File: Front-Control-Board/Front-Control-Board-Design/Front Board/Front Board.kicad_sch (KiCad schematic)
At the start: 27 parts, among them J1 Conn_01x14, J2 Conn_01x14, J3 Conn_01x08, Q1 2N7002, U1 MAX33054EASA+T, U2 TS2940CP33_ROG, U3 ESP32-DevKitC

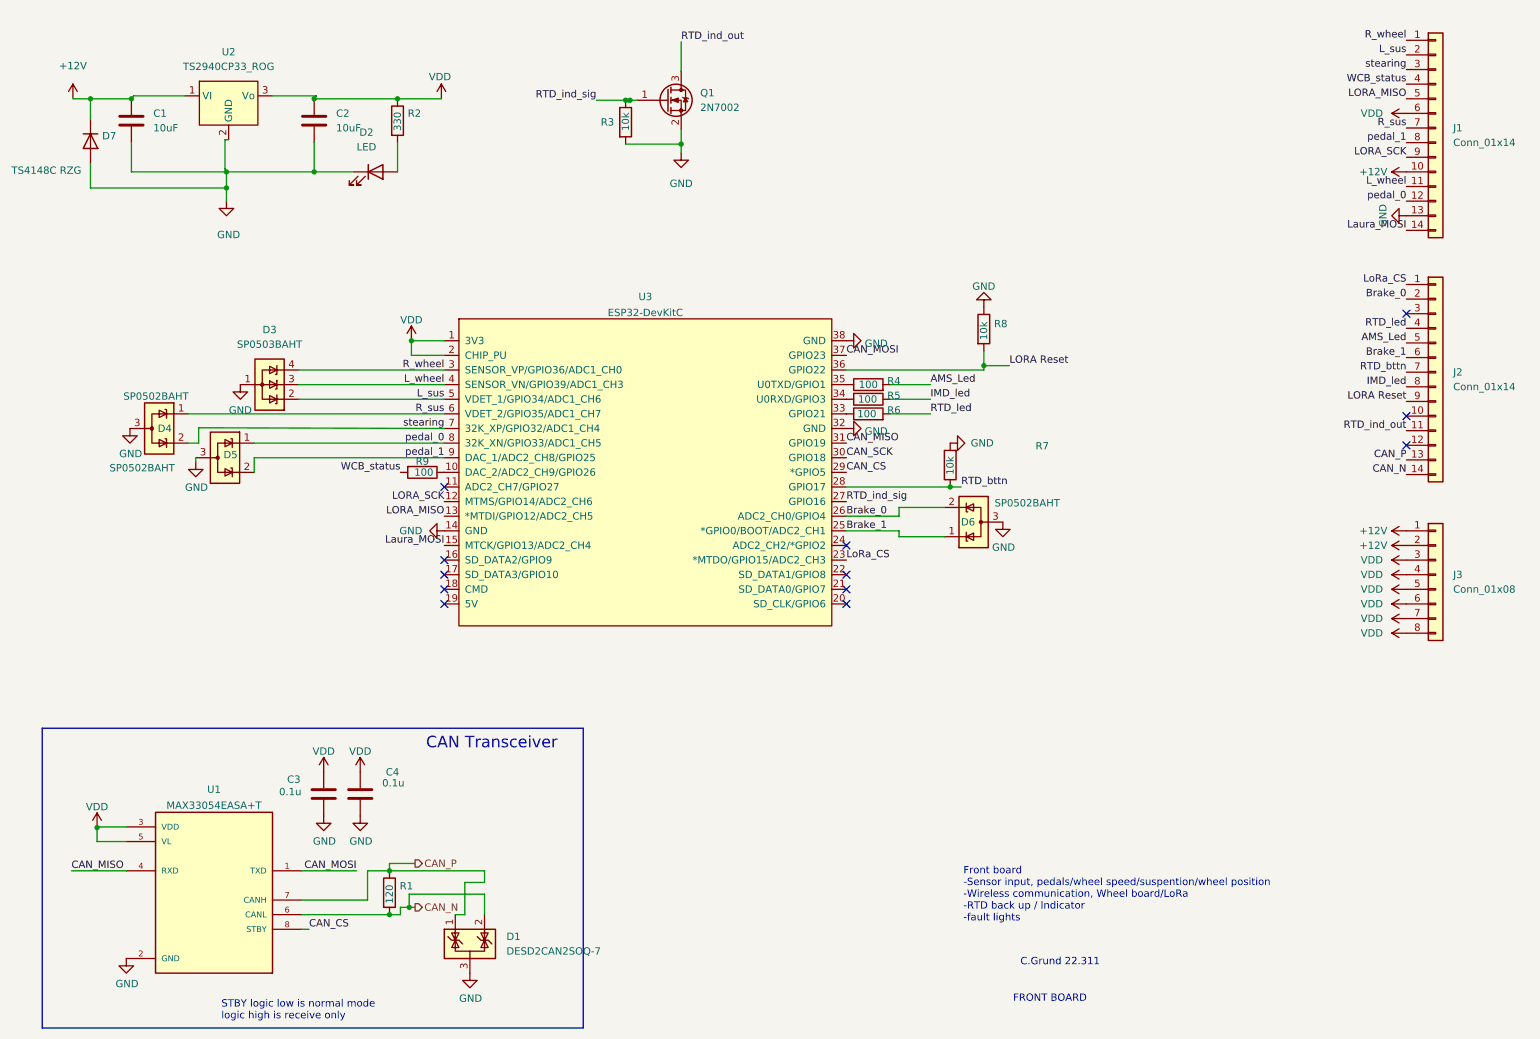
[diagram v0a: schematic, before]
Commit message: end of year DUMP
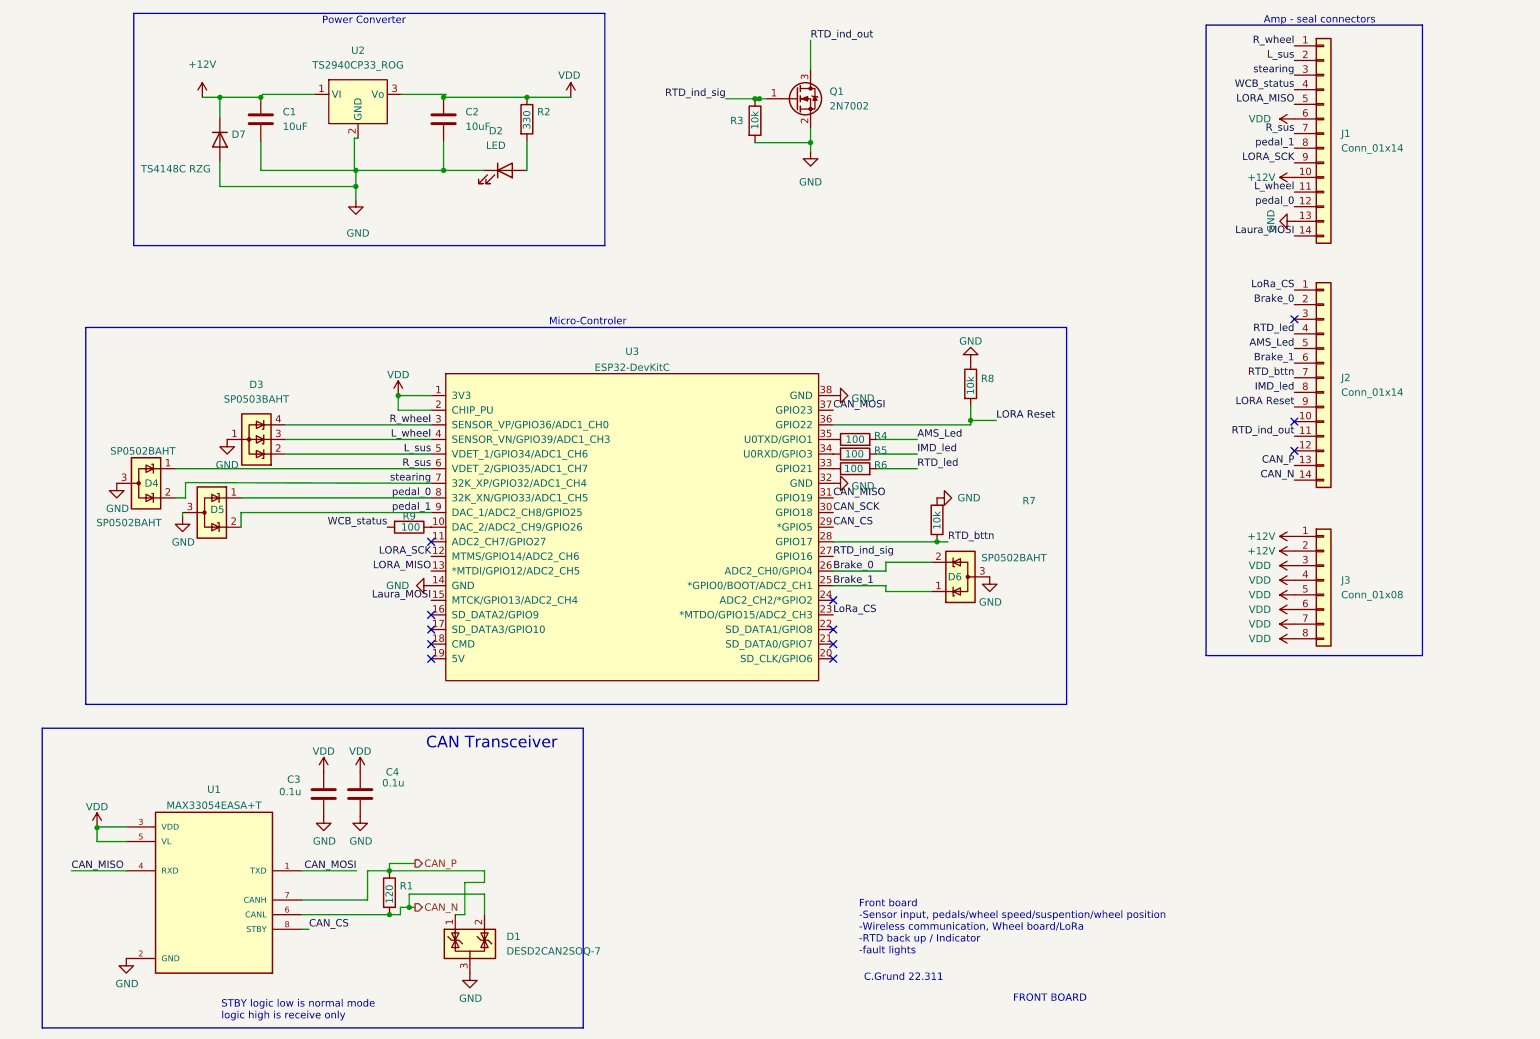
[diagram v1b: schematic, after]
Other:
- note added: "Amp - seal connectors"
- note added: "Micro-Controler"
- note added: "Power Converter"
- moved on the sheet: C1, C2, D2, D3, D4, D5, D6, D7, J1, J2, J3, Q1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
